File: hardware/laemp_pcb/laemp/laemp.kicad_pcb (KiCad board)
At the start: 2 copper layers, 1 part

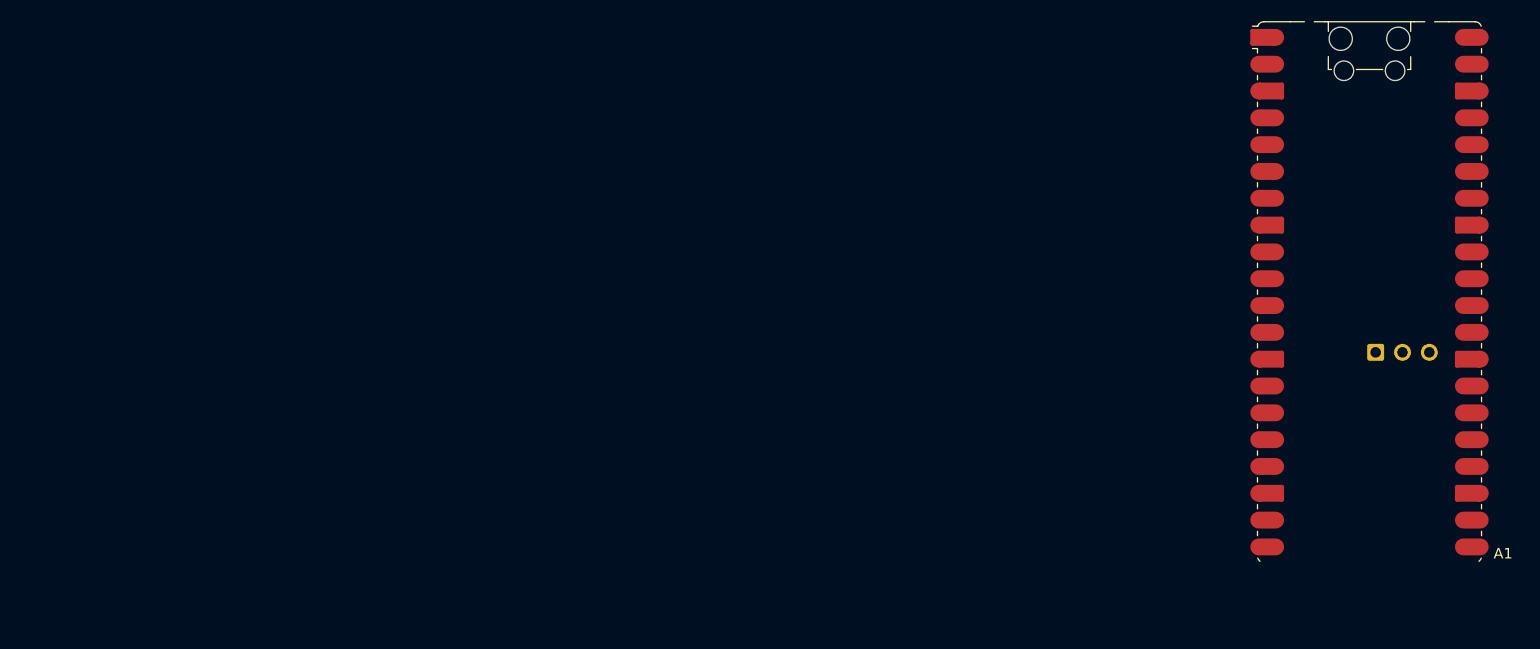
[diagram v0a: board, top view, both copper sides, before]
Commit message: added new lib and schematic changes
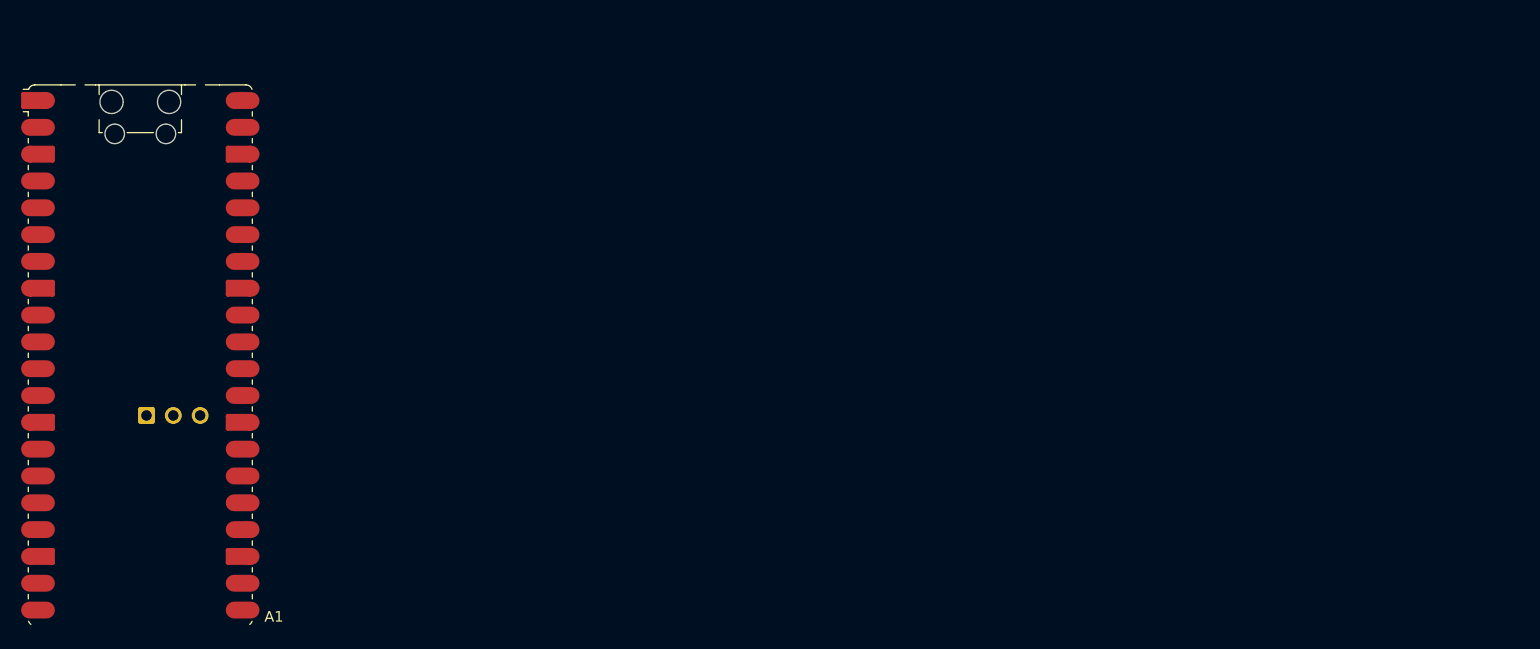
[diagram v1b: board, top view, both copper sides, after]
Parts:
- moved A1 116.6 mm to (75.4, 92.8)
